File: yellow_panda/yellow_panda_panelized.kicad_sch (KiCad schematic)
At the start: 21 parts, among them P1 USB_C_Plug_USB2.0, P2 USB_C_Plug_USB2.0, U1 LT1963AxST-3.3, U2 LT1963AxST-3.3, U5 USBLC6-2SC6, U6 USBLC6-2SC6, U9 TPS2115ADRBR

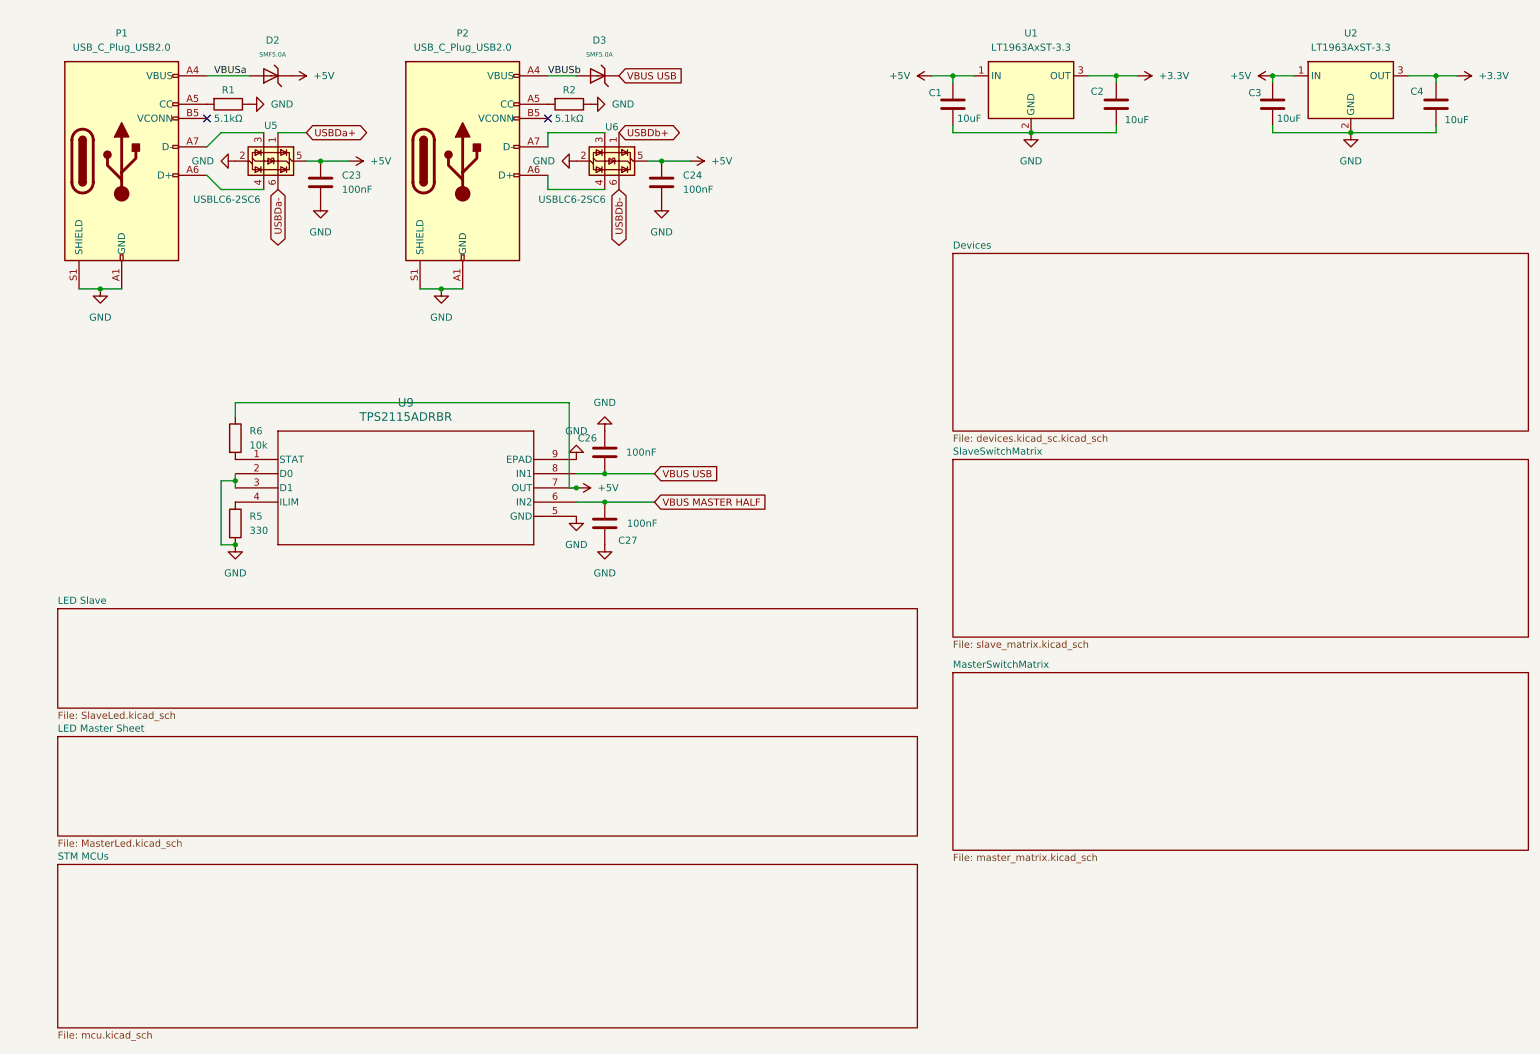
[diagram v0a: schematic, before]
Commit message: v0.1b
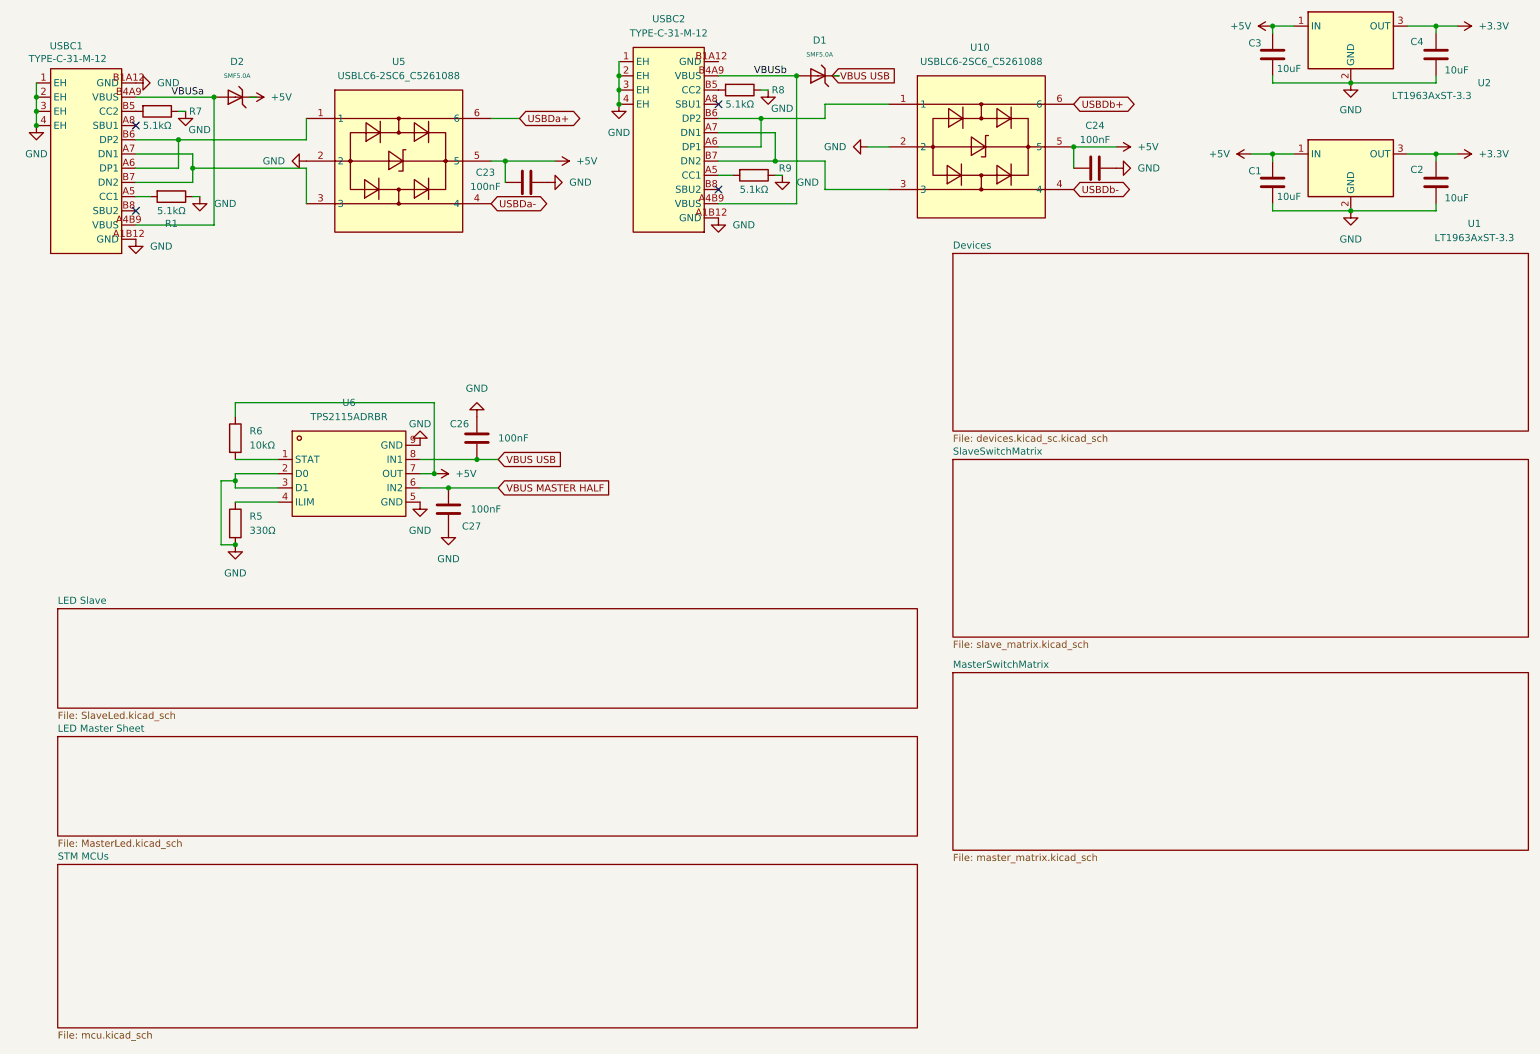
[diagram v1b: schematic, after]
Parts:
- removed D3: SMF5.0A, PCM_JLCPCB:D_SOD-123FL, symbol PCM_JLCPCB-Diodes:TVS-Uni,SMF5.0A
- removed P1, P2: USB_C_Plug_USB2.0, Custom Lib:USB_C_Receptacle_GCT_USB4110, symbol Connector:USB_C_Plug_USB2.0
- removed R2: 5.1kΩ, Resistor_SMD:R_01005_0402Metric_Pad0.57x0.30mm_HandSolder, symbol Device:R
- removed U5, U6: USBLC6-2SC6, Package_TO_SOT_SMD:SOT-23-6, symbol Power_Protection:USBLC6-2SC6
- removed U9: TPS2115ADRBR, Custom Lib:DRB8_2P4X1P65, symbol power_selector:TPS2115ADRBR
- added D1: SMF5.0A, PCM_JLCPCB:D_SOD-123FL, symbol PCM_JLCPCB-Diodes:TVS-Uni,SMF5.0A
- added R7, R8, R9: 5.1kΩ, Resistor_SMD:R_0603_1608Metric, symbol Device:R
- added U10, U5: USBLC6-2SC6_C5261088, easyeda2kicad:SOT-23-6_L2.9-W1.6-P0.95-LS2.8-BR, symbol easyeda2kicad:USBLC6-2SC6_C5261088
- added U6: TPS2115ADRBR, easyeda2kicad:SON-8_L3.0-W3.0-P0.65-LS3.0-BL-EP, symbol easyeda2kicad:TPS2115ADRBR
- added USBC1, USBC2: TYPE-C-31-M-12, easyeda2kicad:USB-C_SMD-TYPE-C-31-M-12_1, symbol easyeda2kicad:TYPE-C-31-M-12
- C1, C2, C3, C4: footprint Capacitor_SMD:C_1206_3216Metric_Pad1.33x1.80mm_HandSolder -> Capacitor_SMD:C_1206_3216Metric; LCSC (none) -> C13585; LCSC Part (none) -> C13585
- C23, C24, C26, C27: footprint Capacitor_SMD:C_0201_0603Metric_Pad0.64x0.40mm_HandSolder -> Capacitor_SMD:C_0805_2012Metric; LCSC (none) -> C48579599; LCSC Part (none) -> C48579599
- D2: LCSC Part (none) -> C19077497
- R1: footprint Resistor_SMD:R_01005_0402Metric_Pad0.57x0.30mm_HandSolder -> Resistor_SMD:R_0603_1608Metric; LCSC (none) -> C2907114; LCSC Part (none) -> C2907114
- R5: value 330 -> 330Ω; footprint Resistor_SMD:R_2512_6332Metric_Pad1.40x3.35mm_HandSolder -> Resistor_SMD:R_0805_2012Metric; LCSC (none) -> C17630; LCSC Part (none) -> C17630
- R6: value 10k -> 10kΩ; footprint Resistor_SMD:R_0402_1005Metric_Pad0.72x0.64mm_HandSolder -> Resistor_SMD:R_0805_2012Metric; LCSC (none) -> C84376; LCSC Part (none) -> C84376
- U1, U2: LCSC (none) -> C6186; LCSC Part (none) -> C6186
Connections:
- net +5V: now also U10.5, U5.5, U6.7 (OUT)
- net GND: now also R7.1, R8.1, R9.1, U10.2, U5.2, U6.2 (D0), U6.3 (D1), U6.5 (GND), U6.9 (GND), USBC1.1 (EH), USBC1.2 (EH), USBC1.3 (EH), USBC1.4 (EH), USBC1.A1B12 (GND), USBC1.B1A12 (GND), USBC2.1 (EH), USBC2.2 (EH), USBC2.3 (EH), USBC2.4 (EH), USBC2.A1B12 (GND)
- net USBDa+: now also U5.6
- net USBDa-: now also U5.4
- net USBDb+: now also U10.6
- net USBDb-: now also U10.4
- net VBUS MASTER HALF: now also U6.6 (IN2)
- net VBUS USB: now also D1.1, U6.8 (IN1)
- net VBUSa: now also USBC1.A4B9 (VBUS), USBC1.B4A9 (VBUS)
- net VBUSb: now also D1.2, USBC2.A4B9 (VBUS), USBC2.B4A9 (VBUS)
- net at R5.1: now also U6.4 (ILIM)
- net at R1.2: now also USBC1.A5 (CC1)
- net at R6.2: now also U6.1 (STAT)
- new net: R9.2, USBC2.A5 (CC1)
- new net: U10.1, USBC2.A6 (DP1), USBC2.B6 (DP2)
- new net: U10.3, USBC2.A7 (DN1), USBC2.B7 (DN2)
- new net: R8.2, USBC2.B5 (CC2)
- new net: U5.1, USBC1.A6 (DP1), USBC1.B6 (DP2)
- new net: U5.3, USBC1.A7 (DN1), USBC1.B7 (DN2)
- new net: R7.2, USBC1.B5 (CC2)
- no-connect marks 2 -> 4
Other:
- moved on the sheet: C1, C2, C23, C24, C26, C27, C3, C4, D2, R1, U1, U2
